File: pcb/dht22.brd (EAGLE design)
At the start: 59.4 x 20.3 mm, 4 parts, among them IC2 MEGA328P

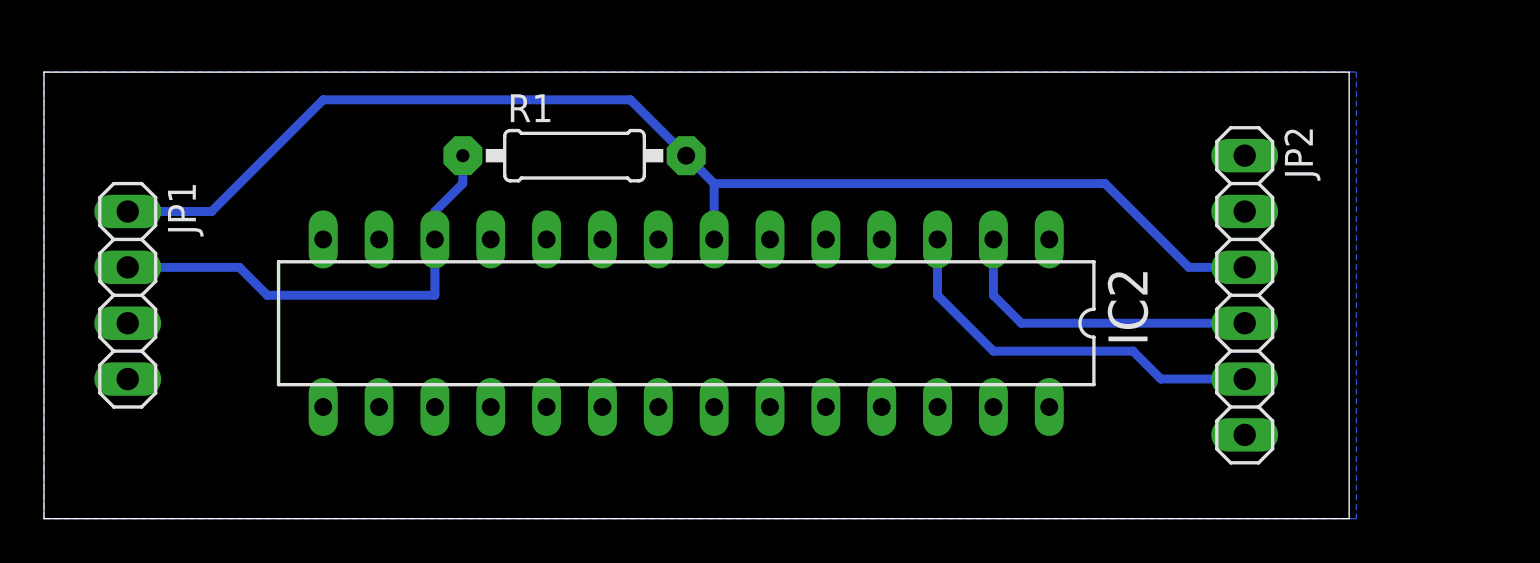
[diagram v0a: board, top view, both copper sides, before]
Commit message: add web
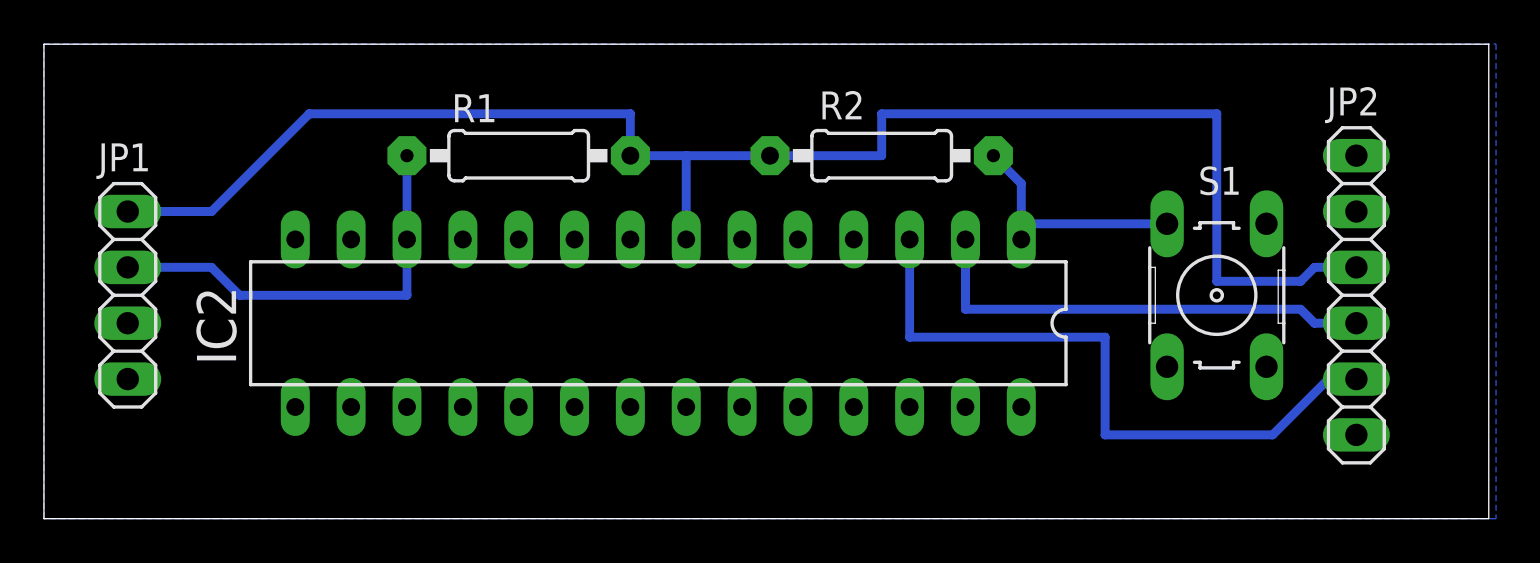
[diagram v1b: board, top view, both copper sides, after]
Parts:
- added R2: 4k7, rcl:0207/10
- added S1: (no value), switch-omron:B3F-10XX
- moved JP2 5.08 mm to (61.0, 10.2)
- moved R1 2.54 mm to (22.9, 16.5)
- moved IC2 1.27 mm to (29.2, 8.89)
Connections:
- new net N$1: IC2.1, R2.1, S1.2
- net GND: now also S1.4
- net VCC: now also R2.2
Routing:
- net VCC: track 58.6 -> 73.2 mm
- net TX: track 18.1 -> 30.3 mm
- net N$1: track 0.00 -> 11.0 mm
- net RX: track 14.5 -> 21.2 mm
- net PD6: track 21.4 -> 19.6 mm
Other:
- board size 59.4 x 20.3 mm -> 65.7 x 21.6 mm
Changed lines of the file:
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@@
 <setting verticaltext="up"/>
 </settings>
-<grid distance="0.05" unitdist="inch" unit="inch" style="lines" multiple="1" display="no" altdistance="0.025" altunitdist="inch" altunit="inch"/>
+<grid distance="25" unitdist="mil" unit="mm" style="lines" multiple="1" display="no" altdistance="0.025" altunitdist="inch" altunit="inch"/>
 <layers>
 <layer number="1" name="Top" color="4" fill="1" visible="yes" active="yes"/>
@@
 <board>
 <plain>
-<wire x1="1.27" y1="0" x2="60.63" y2="0" width="0" layer="20"/>
-<wire x1="60.63" y1="0" x2="60.63" y2="20.31" width="0" layer="20"/>
-<wire x1="60.63" y1="20.31" x2="1.27" y2="20.31" width="0" layer="20"/>
-<wire x1="1.27" y1="20.31" x2="1.27" y2="0" width="0" layer="20"/>
+<wire x1="1.27" y1="0" x2="66.98" y2="0" width="0" layer="20"/>
+<wire x1="66.98" y1="0" x2="66.98" y2="21.58" width="0" layer="20"/>
+<wire x1="66.98" y1="21.58" x2="1.27" y2="21.58" width="0" layer="20"/>
+<wire x1="1.27" y1="21.58" x2="1.27" y2="0" width="0" layer="20"/>
 </plain>
 <attributes>
@@
 </autorouter>
 <elements>
-<element name="JP1" library="pinhead" package="1X04" value="" x="5.08" y="10.16" rot="R270"/>
-<element name="R1" library="rcl" package="0207/10" value="4k7" x="25.4" y="16.51"/>
-<element name="IC2" library="atmel" package="DIL28-3" value="MEGA328P" x="30.48" y="8.89" rot="R180">
-<attribute name="OC_NEWARK" value="unknown" x="30.48" y="8.89" size="1.778" layer="27" rot="R180" display="off"/>
-<attribute name="MPN" value="" x="30.48" y="8.89" size="1.778" layer="27" rot="R180" display="off"/>
-<attribute name="MF" value="" x="30.48" y="8.89" size="1.778" layer="27" rot="R180" display="off"/>
-<attribute name="OC_FARNELL" value="unknown" x="30.48" y="8.89" size="1.778" layer="27" rot="R180" display="off"/>
-</element>
-<element name="JP2" library="pinhead" package="1X06" value="" x="55.88" y="10.16" rot="R270"/>
+<element name="JP1" library="pinhead" package="1X04" value="" x="5.08" y="10.16" smashed="yes" rot="R270">
+<attribute name="NAME" x="3.7338" y="15.7988" size="1.27" layer="25" ratio="10"/>
+<attribute name="VALUE" x="1.905" y="15.24" size="1.27" layer="27" rot="R270"/>
+</element>
+<element name="R1" library="rcl" package="0207/10" value="4k7" x="22.86" y="16.51" smashed="yes">
+<attribute name="NAME" x="19.812" y="18.034" size="1.27" layer="25" ratio="10"/>
+<attribute name="VALUE" x="21.8694" y="15.875" size="1.27" layer="27" ratio="10"/>
+</element>
+<element name="IC2" library="atmel" package="DIL28-3" value="MEGA328P" x="29.21" y="8.89" smashed="yes" rot="R180">
+<attribute name="OC_NEWARK" value="unknown" x="29.21" y="8.89" size="1.778" layer="27" rot="R180" display="off"/>
+<attribute name="MPN" value="" x="29.21" y="8.89" size="1.778" layer="27" rot="R180" display="off"/>
+<attribute name="MF" value="" x="29.21" y="8.89" size="1.778" layer="27" rot="R180" display="off"/>
+<attribute name="OC_FARNELL" value="unknown" x="29.21" y="8.89" size="1.778" layer="27" rot="R180" display="off"/>
+<attribute name="NAME" x="10.0076" y="6.985" size="1.778" layer="25" ratio="10" rot="R90"/>
+<attribute name="VALUE" x="36.195" y="9.525" size="1.778" layer="27" ratio="10" rot="R180"/>
+</element>
+<element name="JP2" library="pinhead" package="1X06" value="" x="60.96" y="10.16" smashed="yes" rot="R270">
+<attribute name="NAME" x="59.6138" y="18.3388" size="1.27" layer="25" ratio="10"/>
+<attribute name="VALUE" x="57.785" y="17.78" size="1.27" layer="27" rot="R270"/>
+</element>
+<element name="S1" library="switch-omron" package="B3F-10XX" value="" x="54.61" y="10.16" smashed="yes" rot="R90">
+<attribute name="OC_NEWARK" value="36M3542" x="54.61" y="10.16" size="1.778" layer="27" rot="R90" display="off"/>
+<attribute name="MPN" value="B3F-1000" x="54.61" y="10.16" size="1.778" layer="27" rot="R90" display="off"/>
+<attribute name="MF" value="" x="54.61" y="10.16" size="1.778" layer="27" rot="R90" display="off"/>
+<attribute name="OC_FARNELL" value="176432" x="54.61" y="10.16" size="1.778" layer="27" rot="R90" display="off"/>
+<attribute name="NAME" x="55.753" y="16.002" size="1.27" layer="25" ratio="10" rot="R180"/>
+<attribute name="VALUE" x="59.69" y="7.112" size="1.27" layer="27" ratio="10" rot="R90"/>
+</element>
+<element name="R2" library="rcl" package="0207/10" value="4k7" x="39.37" y="16.51" smashed="yes" rot="R180">
+<attribute name="NAME" x="38.608" y="19.431" size="1.27" layer="25" ratio="10" rot="R180"/>
+<attribute name="VALUE" x="40.9956" y="17.145" size="1.27" layer="27" ratio="10" rot="R180"/>
+</element>
 </elements>
 <signals>
@@
 <contactref element="JP2" pad="3"/>
 <wire x1="5.08" y1="13.97" x2="8.89" y2="13.97" width="0.4064" layer="16"/>
-<wire x1="55.88" y1="11.43" x2="53.34" y2="11.43" width="0.4064" layer="16"/>
-<wire x1="53.34" y1="11.43" x2="49.53" y2="15.24" width="0.4064" layer="16"/>
-<wire x1="49.53" y1="15.24" x2="31.75" y2="15.24" width="0.4064" layer="16"/>
-<wire x1="31.75" y1="15.24" x2="31.75" y2="12.7" width="0.4064" layer="16"/>
-<wire x1="30.48" y1="16.51" x2="31.75" y2="15.24" width="0.4064" layer="16"/>
-<wire x1="8.89" y1="13.97" x2="13.97" y2="19.05" width="0.4064" layer="16"/>
-<wire x1="13.97" y1="19.05" x2="27.94" y2="19.05" width="0.4064" layer="16"/>
-<wire x1="27.94" y1="19.05" x2="30.48" y2="16.51" width="0.4064" layer="16"/>
+<wire x1="30.48" y1="16.51" x2="30.48" y2="12.7" width="0.4064" layer="16"/>
+<wire x1="27.94" y1="16.51" x2="30.48" y2="16.51" width="0.4064" layer="16"/>
+<wire x1="8.89" y1="13.97" x2="13.335" y2="18.415" width="0.4064" layer="16"/>
+<wire x1="13.335" y1="18.415" x2="27.94" y2="18.415" width="0.4064" layer="16"/>
+<wire x1="27.94" y1="18.415" x2="27.94" y2="16.51" width="0.4064" layer="16"/>
+<contactref element="R2" pad="2"/>
+<wire x1="34.29" y1="16.51" x2="30.48" y2="16.51" width="0.4064" layer="16"/>
+<wire x1="34.29" y1="16.51" x2="39.37" y2="16.51" width="0.4064" layer="16"/>
+<wire x1="39.37" y1="16.51" x2="39.37" y2="18.415" width="0.4064" layer="16"/>
+<wire x1="60.96" y1="11.43" x2="59.055" y2="11.43" width="0.4064" layer="16"/>
+<wire x1="59.055" y1="11.43" x2="58.42" y2="10.795" width="0.4064" layer="16"/>
+<wire x1="58.42" y1="10.795" x2="54.61" y2="10.795" width="0.4064" layer="16"/>
+<wire x1="54.61" y1="10.795" x2="54.61" y2="18.415" width="0.4064" layer="16"/>
+<wire x1="54.61" y1="18.415" x2="39.37" y2="18.415" width="0.4064" layer="16"/>
 </signal>
 <signal name="GND">
@@
 <contactref element="JP2" pad="2"/>
 <polygon width="0.4064" layer="16" isolate="0.6096">
-<vertex x="1.27" y="20.32"/>
-<vertex x="60.96" y="20.32"/>
-<vertex x="60.96" y="0"/>
+<vertex x="1.27" y="21.59"/>
+<vertex x="67.31" y="21.59"/>
+<vertex x="67.31" y="0"/>
 <vertex x="1.27" y="0"/>
 </polygon>
+<contactref element="S1" pad="4"/>
 </signal>
 <signal name="PD6">
@@
 <contactref element="JP1" pad="2"/>
 <contactref element="R1" pad="1"/>
-<wire x1="5.08" y1="11.43" x2="10.16" y2="11.43" width="0.4064" layer="16"/>
-<wire x1="10.16" y1="11.43" x2="11.43" y2="10.16" width="0.4064" layer="16"/>
-<wire x1="11.43" y1="10.16" x2="19.05" y2="10.16" width="0.4064" layer="16"/>
-<wire x1="19.05" y1="10.16" x2="19.05" y2="12.7" width="0.4064" layer="16"/>
-<wire x1="20.32" y1="16.51" x2="20.32" y2="15.24" width="0.4064" layer="16"/>
-<wire x1="20.32" y1="15.24" x2="19.05" y2="13.97" width="0.4064" layer="16"/>
-<wire x1="19.05" y1="13.97" x2="19.05" y2="12.7" width="0.4064" layer="16"/>
+<wire x1="5.08" y1="11.43" x2="8.89" y2="11.43" width="0.4064" layer="16"/>
+<wire x1="8.89" y1="11.43" x2="10.16" y2="10.16" width="0.4064" layer="16"/>
+<wire x1="10.16" y1="10.16" x2="17.78" y2="10.16" width="0.4064" layer="16"/>
+<wire x1="17.78" y1="10.16" x2="17.78" y2="12.7" width="0.4064" layer="16"/>
+<wire x1="17.78" y1="16.51" x2="17.78" y2="12.7" width="0.4064" layer="16"/>
 </signal>
 <signal name="RX">
 <contactref element="IC2" pad="2"/>
 <contactref element="JP2" pad="4"/>
-<wire x1="44.45" y1="12.7" x2="44.45" y2="10.16" width="0.4064" layer="16"/>
-<wire x1="44.45" y1="10.16" x2="45.72" y2="8.89" width="0.4064" layer="16"/>
-<wire x1="45.72" y1="8.89" x2="55.88" y2="8.89" width="0.4064" layer="16"/>
+<wire x1="43.18" y1="12.7" x2="43.18" y2="9.525" width="0.4064" layer="16"/>
+<wire x1="43.18" y1="9.525" x2="58.42" y2="9.525" width="0.4064" layer="16"/>
+<wire x1="58.42" y1="9.525" x2="59.055" y2="8.89" width="0.4064" layer="16"/>
+<wire x1="59.055" y1="8.89" x2="60.96" y2="8.89" width="0.4064" layer="16"/>
 </signal>
 <signal name="TX">
 <contactref element="IC2" pad="3"/>
 <contactref element="JP2" pad="5"/>
-<wire x1="41.91" y1="12.7" x2="41.91" y2="10.16" width="0.4064" layer="16"/>
-<wire x1="41.91" y1="10.16" x2="44.45" y2="7.62" width="0.4064" layer="16"/>
-<wire x1="44.45" y1="7.62" x2="50.8" y2="7.62" width="0.4064" layer="16"/>
-<wire x1="50.8" y1="7.62" x2="52.07" y2="6.35" width="0.4064" layer="16"/>
-<wire x1="52.07" y1="6.35" x2="55.88" y2="6.35" width="0.4064" layer="16"/>
+<wire x1="49.53" y1="8.255" x2="49.53" y2="3.81" width="0.4064" layer="16"/>
+<wire x1="49.53" y1="3.81" x2="57.15" y2="3.81" width="0.4064" layer="16"/>
+<wire x1="57.15" y1="3.81" x2="59.69" y2="6.35" width="0.4064" layer="16"/>
+<wire x1="59.69" y1="6.35" x2="60.96" y2="6.35" width="0.4064" layer="16"/>
+<wire x1="40.64" y1="12.7" x2="40.64" y2="8.255" width="0.4064" layer="16"/>
+<wire x1="40.64" y1="8.255" x2="49.53" y2="8.255" width="0.4064" layer="16"/>
+</signal>
+<signal name="N$1">
+<contactref element="IC2" pad="1"/>
+<contactref element="S1" pad="2"/>
+<contactref element="R2" pad="1"/>
+<wire x1="44.45" y1="16.51" x2="45.72" y2="15.24" width="0.4064" layer="16"/>
+<wire x1="45.72" y1="15.24" x2="45.72" y2="13.335" width="0.4064" layer="16"/>
+<wire x1="45.72" y1="13.335" x2="45.72" y2="12.7" width="0.4064" layer="16"/>
+<wire x1="52.3494" y1="13.4112" x2="45.7962" y2="13.4112" width="0.4064" layer="16"/>
+<wire x1="45.7962" y1="13.4112" x2="45.72" y2="13.335" width="0.4064" layer="16"/>
 </signal>
 </signals>
